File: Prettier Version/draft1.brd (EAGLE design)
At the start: 160 x 100 mm, 27 parts, among them J1 USB_MICRO_AB, J2 CONN-51P-FPC-MOLEX, J4 DISPLAYPORT-SINK-MOLEX, Q1 Si2304, U1 ESD-SUPPRESSOR-4-TPD4S010-DQA, U2 ESD-SUPPRESSOR-4-TPD4S010-DQA, U3 ESD-SUPPRESSOR-4-TPD4S010-DQA, U4 MAX8790A-TQFN-20

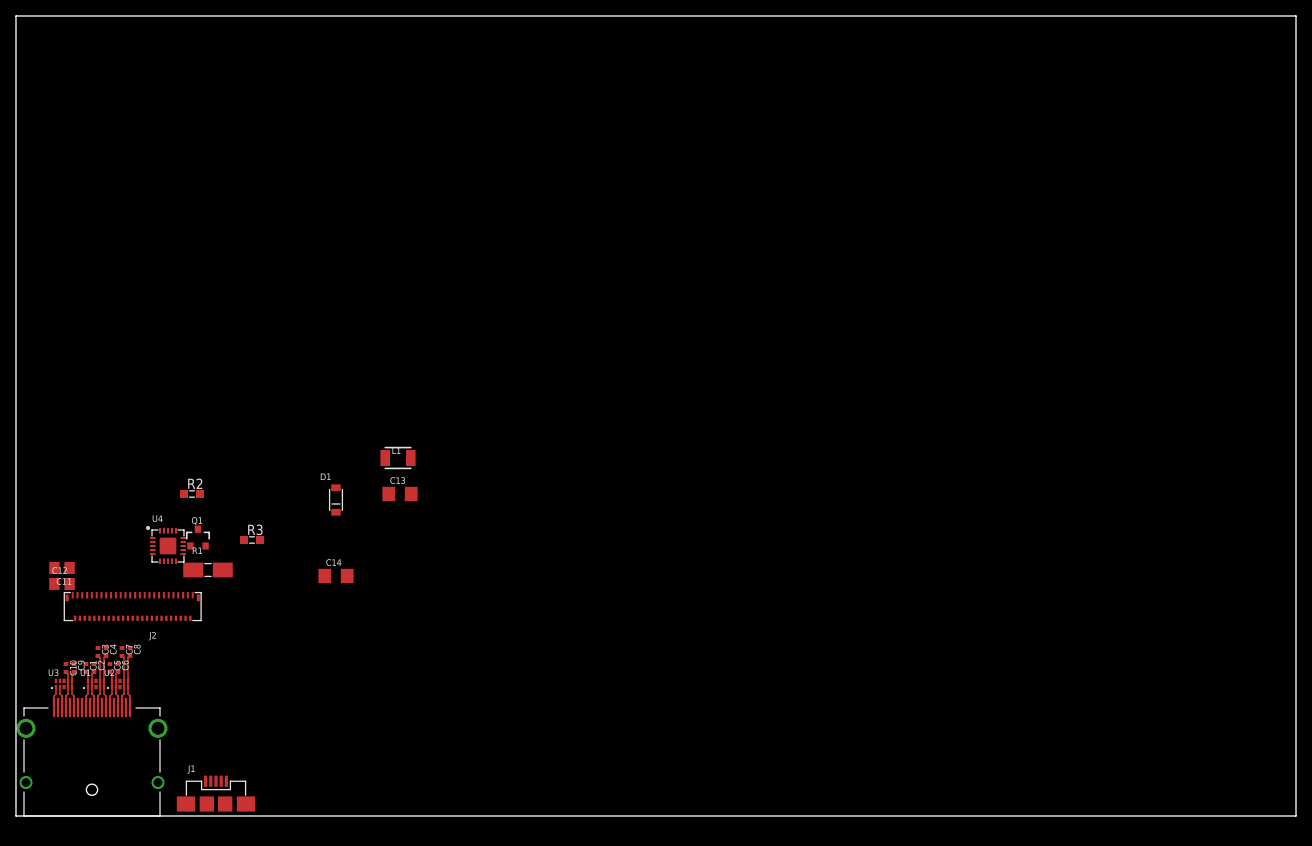
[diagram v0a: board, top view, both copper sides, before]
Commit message: Prelim. PCB layout
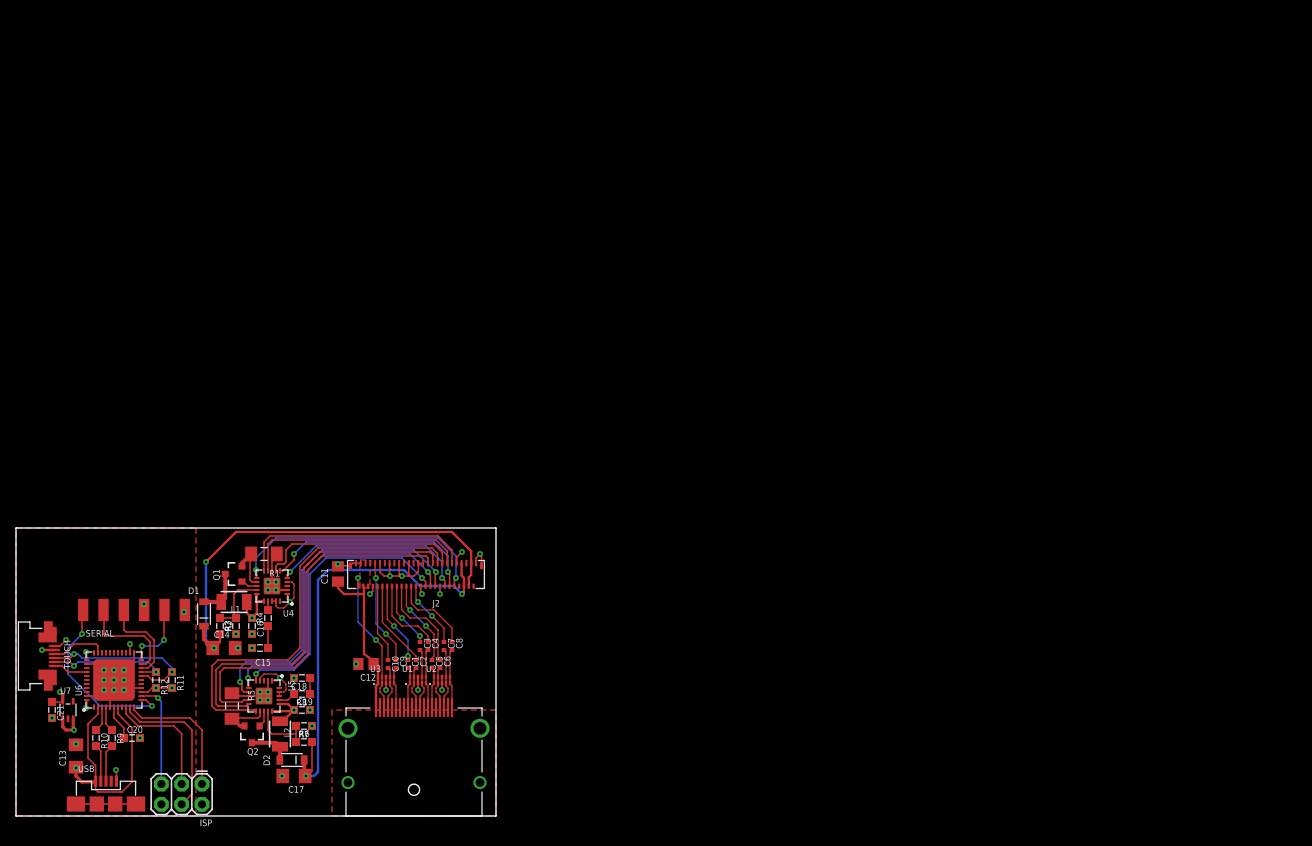
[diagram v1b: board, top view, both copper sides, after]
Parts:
- removed J1: USB_MICRO_AB, 00-EvaLibrary:USB_MICRO_AB
- removed J4: DISPLAYPORT-SINK-MOLEX, 00-EvaLibrary:MOLEX-47272-0028
- added C15, C18: 0.1u, 00-EvaLibrary:C0603
- added C16, C19, C20, C21: 1u, 00-EvaLibrary:C0603
- added C17: 2.2u, 00-EvaLibrary:C1206
- added D2: DB2W40300L, 00-EvaLibrary:MINI2-F3-B
- added DP: DISPLAYPORT-SINK-MOLEX, 00-EvaLibrary:MOLEX-47272-0028
- added ISP: AVR_SPI_PRG_6PTH, SparkFun-Connectors:2X3
- added L2: 2.2u, 00-EvaLibrary:1210
- added Q2: Si2304, SparkFun-DiscreteSemi:SOT23-3
- added R10, R9: 22, 00-EvaLibrary:R0603
- added R11, R12: 4.7K, 00-EvaLibrary:R0603
- added R4, R8: 1.2K, 00-EvaLibrary:R0603
- added R5: 50m, 00-EvaLibrary:MCS1632
- added R6: 1M, 00-EvaLibrary:R0603
- added R7: 43.2K, 00-EvaLibrary:R0603
- added SERIAL: HEADER-6X1-961106-5500, 00-EvaLibrary:HEADER-3M-961-6P-2.54MM
- added TOUCH: HEADER-6X1-FPC-LOWER_CONTACT, 00-EvaLibrary:SFV6R-1STE1HLF
- added U5: MAX8790A-TQFN-20, 00-EvaLibrary:TQFN-20
- added U6: ATMEGA32U4-QFN-44, 00-EvaLibrary:QFN-44
- added U7: TLV700DDC, 00-EvaLibrary:SOT-23-5
- added USB: USB_MICRO_AB, 00-EvaLibrary:USB_MICRO_AB
- moved C13 52.1 mm to (7.50, 7.50), turned to 90 degrees
- moved C3 40.3 mm to (50.5, 21.2)
- moved C4 40.3 mm to (51.5, 21.2)
- moved C7 40.3 mm to (53.5, 21.2)
- moved C8 40.3 mm to (54.5, 21.2)
- moved C1 40.3 mm to (49.0, 19.0)
- moved C10 40.3 mm to (46.5, 19.0)
- moved C2 40.3 mm to (50.0, 19.0)
- moved C5 40.3 mm to (52.0, 19.0)
- moved C6 40.3 mm to (53.0, 19.0)
- moved C9 40.3 mm to (47.5, 19.0)
- moved U1 40.3 mm to (50.2, 17.0)
- moved U2 40.3 mm to (53.2, 17.0)
- moved U3 40.3 mm to (46.2, 17.0)
- moved C12 39.3 mm to (43.8, 19.0), turned to 180 degrees
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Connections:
- new net !RESET: ISP.5, U6.13
- new net BRIGHTNESS1: U4.3
- new net BRIGHTNESS2: U5.3
- new net CTS: SERIAL.5, U6.22
- new net D+: R9.2, USB.3
- new net D-: R10.2, USB.2
- new net D3.3V: C21.1, R11.2, R12.2, TOUCH.5, U6.14, U6.24, U6.34, U6.44, U7.5
- new net INT: TOUCH.4, U6.32
- new net MISO: ISP.1, U6.11
- new net MOSI: ISP.4, U6.10
- new net N$16: R4.2, U4.17
- new net N$17: C15.1, R4.1
- new net N$18: D2.2, L2.2, Q2.3
- new net N$19: Q2.2, R5.2, U5.12
- new net N$20: R6.1, R7.2, U5.14
- new net N$21: R8.2, U5.17
- new net N$22: C18.1, R8.1
- new net N$23: R9.1, U6.4
- new net N$24: R10.1, U6.3
- new net N$25: C20.1, U6.6
- new net RTS: SERIAL.1, U6.12
- new net RXD: SERIAL.3, U6.20
- new net SCL: R11.1, TOUCH.3, U6.18
- new net SCLK: ISP.3, U6.9
- new net SCREEN_!RESET: TOUCH.1, U6.37
- new net SDA: R12.1, TOUCH.2, U6.19
- new net TXD: SERIAL.2, U6.21
- new net VBUS: C13.1, C16.1, C19.1, ISP.2, L1.1, L2.1, SERIAL.4, U4.1, U4.15, U4.16, U4.18, U4.19, U4.4, U5.1, U5.15, U5.16, U5.18, U5.19, U5.4, U6.2, U6.7, U7.1, U7.3, USB.1
- net 3.3V: now also DP.20; no longer J4.20
- net GND: now also C15.2, C16.2, C17.2, C18.2, C19.2, C20.2, C21.2, DP.11, DP.16, DP.19, DP.2, DP.5, DP.8, DP.GND1, DP.GND2, DP.GND3, DP.GND4, ISP.6, R5.1, R7.1, SERIAL.6, TOUCH.6, U4.2, U5.2, U5.8, U5.PAD, U6.15, U6.23, U6.35, U6.43, U6.5, U6.PAD, U7.2, USB.5, USB.GND1, USB.GND2, USB.GND3, USB.GND4; no longer J1.5, J1.GND1, J1.GND2, J1.GND3, J1.GND4, J4.11, J4.16, J4.19, J4.2, J4.5, J4.8, J4.GND1, J4.GND2, J4.GND3, J4.GND4
- net HPD: now also DP.18; no longer J4.18
- net LED_A2: now also C17.1, D2.1, R6.2
- net LED_K1B: now also U5.11
- net LED_K2B: now also U5.7
- net LED_K3A: now also U4.6; no longer U4.9
- net LED_K3B: now also U5.10
- net LED_K4A: now also U4.9; no longer U4.7
- net LED_K4B: now also U5.6
- net LED_K5A: now also U4.5; no longer U4.6
- net LED_K5B: now also U5.9
- net LED_K6A: now also U4.7; no longer U4.5
- net LED_K6B: now also U5.5
- net N$1: now also DP.7; no longer J4.7
- net N$10: now also DP.17; no longer J4.17
- net N$12: now also Q2.1, U5.13; no longer C13.1, J1.1, L1.1, U4.1, U4.15, U4.16, U4.18, U4.4
- net N$2: now also DP.9; no longer J4.9
- net N$3: now also DP.10; no longer J4.10
- net N$4: now also DP.12; no longer J4.12
- net N$5: now also DP.6; no longer J4.6
- net N$6: now also DP.4; no longer J4.4
- net N$7: now also DP.3; no longer J4.3
- net N$8: now also DP.1; no longer J4.1
- net N$9: now also DP.15; no longer J4.15
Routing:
- net GND: track 0.00 -> 74.4 mm, vias 0 -> 43
- net VBUS: track 0.00 -> 65.0 mm, vias 0 -> 7
- net LED_A1: track 0.00 -> 57.1 mm, vias 0 -> 2
- net LED_A2: track 0.00 -> 56.4 mm, vias 0 -> 2
- net LED_K1B: track 0.00 -> 52.6 mm
- net LED_K3B: track 0.00 -> 49.1 mm
- net LED_K5B: track 0.00 -> 46.2 mm
- net LED_K2B: track 0.00 -> 43.2 mm, vias 0 -> 2
- net LED_K4B: track 0.00 -> 39.5 mm, vias 0 -> 2
- net LED_K6B: track 0.00 -> 35.7 mm, vias 0 -> 2
- net LED_K1A: track 0.00 -> 33.3 mm, vias 0 -> 2
- net LED_K2A: track 0.00 -> 29.8 mm
- net LED_K4A: track 0.00 -> 28.0 mm
- net LED_K3A: track 0.00 -> 27.5 mm, vias 0 -> 2
- net LED_K5A: track 0.00 -> 25.2 mm, vias 0 -> 2
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- added copper zone on layer 1, net 3.3V
- added copper zone on layer 3, net D3.3V
- added copper zone on layer 1, net GND
- added copper zone on layer 2, net GND
- added copper zone on layer 3, net GND
- added copper zone on layer 3, net VBUS
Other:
- board size 160 x 100 mm -> 60 x 36 mm
